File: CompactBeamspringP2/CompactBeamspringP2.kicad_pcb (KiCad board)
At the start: 2 copper layers, 163.6 x 33.2 mm, 68 parts, among them J1 BEAMSPRING CONNECTOR, J2 PadsToShort, J3 EXPANSION HEADER, U1 MCP4921-E, U2 LM339A, U3 74AHC595, U4 74AHC595, U5 ProMicro, U7 74AHC595

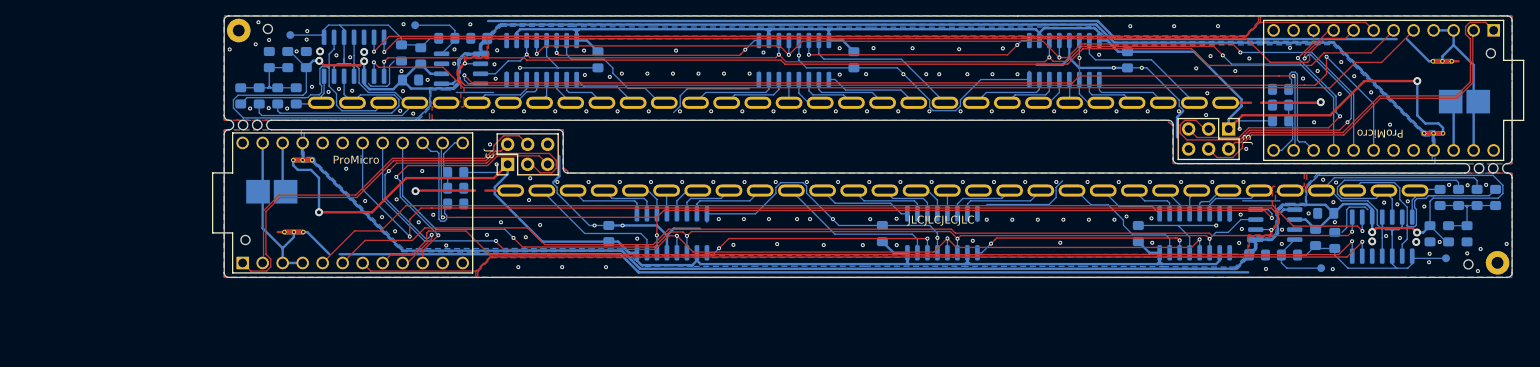
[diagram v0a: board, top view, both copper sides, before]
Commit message: Updated to rev. 1.4
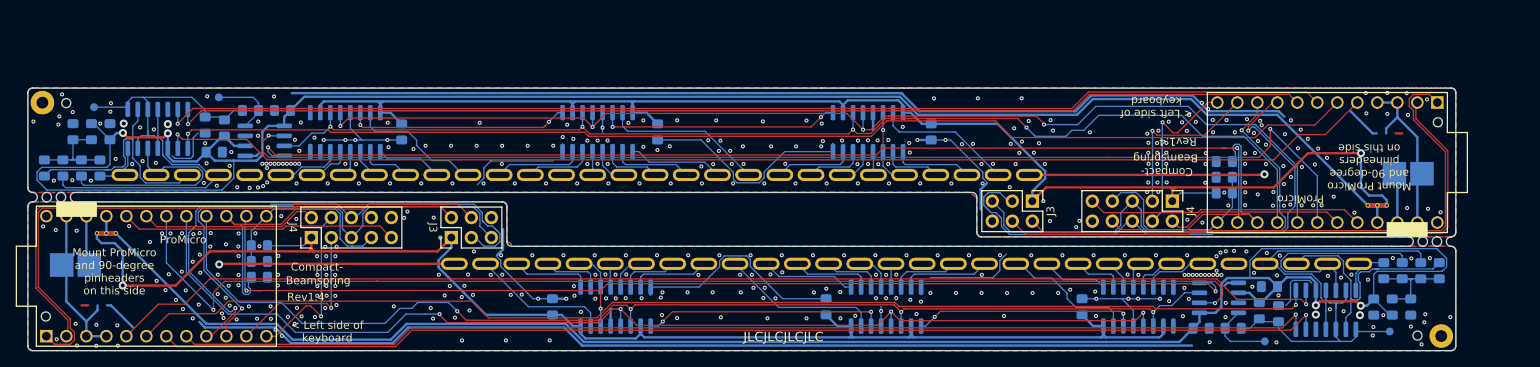
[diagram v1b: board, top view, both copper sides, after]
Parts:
- removed the C1 at (241.3, 128.8)
- removed the C1 at (142.4, 101.2)
- removed the C2 at (158.9, 126.0)
- removed the C2 at (224.8, 104.0)
- removed the C3 at (263.2, 126.1)
- removed the C3 at (120.5, 103.9)
- removed the C4 at (193.6, 126.0)
- removed the C4 at (190.0, 104.0)
- removed the C5 at (226.1, 126.0)
- removed the C5 at (157.5, 104.0)
- removed the C6 at (249.9, 123.5)
- removed the C6 at (133.7, 106.5)
- removed the H1 at (271.8, 129.8)
- removed the H1 at (111.9, 100.2)
- removed the J1 at (203.9, 120.6)
- removed the J1 at (179.8, 109.4)
- removed the J2 at (116.1, 117.8)
- removed the J2 at (267.6, 112.2)
- removed the J3 at (146.0, 117.2)
- removed the J3 at (237.6, 112.8)
- removed NT1 (x2): Net-Tie_3, NetTie:NetTie-3_THT_Pad0.3mm
- removed the NT2 at (118.8, 116.7)
- removed the NT2 at (264.8, 113.3)
- removed the R1 at (265.5, 126.1)
- removed the R1 at (118.1, 103.9)
- removed the R10 at (264.4, 121.5)
- removed the R10 at (119.2, 108.5)
- removed the R11 at (269.1, 121.5)
- removed the R11 at (114.5, 108.5)
- removed the R12 at (271.5, 121.5)
- removed the R12 at (112.2, 108.5)
- removed the R2 at (267.9, 126.1)
- removed the R2 at (115.8, 103.9)
- removed the R3 at (248.6, 126.5)
- removed the R3 at (135.0, 103.5)
- removed the R4 at (245.3, 128.8)
- removed the R4 at (138.3, 101.2)
- removed the R5 at (251.1, 126.9)
- removed the R5 at (132.6, 103.1)
- removed the R6 at (139.4, 118.3)
- removed the R6 at (244.2, 111.7)
- removed the R7 at (139.4, 120.3)
- removed the R7 at (244.2, 109.7)
- removed the R8 at (139.4, 122.3)
- removed the R8 at (244.2, 107.7)
- removed the R9 at (266.8, 121.5)
- removed the R9 at (116.8, 108.5)
- removed REF** (x4): tooling_hole, TH-XWhatsIt:tooling_hole
- removed the TP1 at (249.3, 130.4)
- removed the TP1 at (134.3, 99.6)
- removed the TP2 at (265.2, 129.2)
- removed the TP2 at (118.5, 100.8)
- removed the U1 at (243.5, 124.9)
- removed the U1 at (140.1, 105.1)
- removed the U2 at (257.1, 126.4)
- removed the U2 at (126.5, 103.6)
- removed the U3 at (166.9, 126.0)
- removed the U3 at (216.7, 104.0)
- removed the U4 at (201.3, 126.0)
- removed the U4 at (182.4, 104.0)
- removed the U5 at (126.4, 122.1)
- removed the U5 at (257.3, 107.9)
- removed the U7 at (233.3, 126.0)
- removed the U7 at (150.4, 104.0)
- added C1: 0U1, Capacitor_SMD:C_0805_2012Metric_Pad1.15x1.40mm_HandSolder, B.Cu at (234.1, 138.1)
- added C1: 0U1, Capacitor_SMD:C_0805_2012Metric_Pad1.15x1.40mm_HandSolder, B.Cu at (117.5, 110.4)
- added C2: 0U1, Capacitor_SMD:C_0805_2012Metric_Pad1.15x1.40mm_HandSolder, B.Cu at (151.7, 135.3)
- added C2: 0U1, Capacitor_SMD:C_0805_2012Metric_Pad1.15x1.40mm_HandSolder, B.Cu at (199.8, 113.1)
- added C3: 0U1, Capacitor_SMD:C_0805_2012Metric_Pad1.15x1.40mm_HandSolder, B.Cu at (256.0, 135.4)
- added C3: 0U1, Capacitor_SMD:C_0805_2012Metric_Pad1.15x1.40mm_HandSolder, B.Cu at (95.5, 113.1)
- added C4: 0U1, Capacitor_SMD:C_0805_2012Metric_Pad1.15x1.40mm_HandSolder, B.Cu at (186.5, 135.3)
- added C4: 0U1, Capacitor_SMD:C_0805_2012Metric_Pad1.15x1.40mm_HandSolder, B.Cu at (165.1, 113.1)
- added C5: 0U1, Capacitor_SMD:C_0805_2012Metric_Pad1.15x1.40mm_HandSolder, B.Cu at (219.0, 135.3)
- added C5: 0U1, Capacitor_SMD:C_0805_2012Metric_Pad1.15x1.40mm_HandSolder, B.Cu at (132.6, 113.1)
- added C6: 0U1, Capacitor_SMD:C_0805_2012Metric_Pad1.15x1.40mm_HandSolder, B.Cu at (242.8, 132.8)
- added C6: 0U1, Capacitor_SMD:C_0805_2012Metric_Pad1.15x1.40mm_HandSolder, B.Cu at (108.8, 115.7)
- added H1: MountingHole_Pad, TH-XWhatsIt:ChassisGnd, B.Cu at (264.6, 139.1)
- added H1: MountingHole_Pad, TH-XWhatsIt:ChassisGnd, B.Cu at (87.0, 109.4)
- added H2: ToolingHole, TH-XWhatsIt:tooling_hole, F.Cu at (87.4, 136.6)
- added H2: ToolingHole, TH-XWhatsIt:tooling_hole, F.Cu at (264.2, 111.9)
- added H3: ToolingHole, TH-XWhatsIt:tooling_hole, F.Cu at (261.6, 139.0)
- added H3: ToolingHole, TH-XWhatsIt:tooling_hole, F.Cu at (90.0, 109.5)
- added J1: BEAMSPRING CONNECTOR, TH-XWhatsIt:30-pin-universal-beamspring-connector_v2, F.Cu at (196.7, 129.9)
- added J1: BEAMSPRING CONNECTOR, TH-XWhatsIt:30-pin-universal-beamspring-connector_v2, F.Cu at (154.9, 118.6)
- added J2: PadsToShort, TH-XWhatsIt:PadsToShort, B.Cu at (91.2, 127.1)
- added J2: PadsToShort, TH-XWhatsIt:PadsToShort, B.Cu at (260.4, 121.3)
- added J3: EXPANSION HEADER, Connector_PinHeader_2.54mm:PinHeader_2x03_P2.54mm_Vertical, F.Cu at (138.9, 126.5)
- added J3: EXPANSION HEADER, Connector_PinHeader_2.54mm:PinHeader_2x03_P2.54mm_Vertical, F.Cu at (212.7, 121.9)
- added J4: Conn_02x05_Odd_Even, Connector_PinHeader_2.54mm:PinHeader_2x05_P2.54mm_Vertical, F.Cu at (121.1, 126.5)
- added J4: Conn_02x05_Odd_Even, Connector_PinHeader_2.54mm:PinHeader_2x05_P2.54mm_Vertical, F.Cu at (230.5, 121.9)
- added NT2: Net-Tie_3, NetTie:NetTie-3_THT_Pad0.3mm, B.Cu at (93.9, 126.0)
- added NT2: Net-Tie_3, NetTie:NetTie-3_THT_Pad0.3mm, B.Cu at (257.7, 122.5)
- added R1: 4K7, Resistor_SMD:R_0805_2012Metric_Pad1.15x1.40mm_HandSolder, B.Cu at (258.4, 135.4)
- added R1: 4K7, Resistor_SMD:R_0805_2012Metric_Pad1.15x1.40mm_HandSolder, B.Cu at (93.2, 113.1)
- added R10: 100k 1%, Resistor_SMD:R_0805_2012Metric_Pad1.15x1.40mm_HandSolder, B.Cu at (257.3, 130.8)
- added R10: 100k 1%, Resistor_SMD:R_0805_2012Metric_Pad1.15x1.40mm_HandSolder, B.Cu at (94.3, 117.7)
- added R11: 100k 1%, Resistor_SMD:R_0805_2012Metric_Pad1.15x1.40mm_HandSolder, B.Cu at (262.0, 130.8)
- added R11: 100k 1%, Resistor_SMD:R_0805_2012Metric_Pad1.15x1.40mm_HandSolder, B.Cu at (89.6, 117.7)
- added R12: 100k 1%, Resistor_SMD:R_0805_2012Metric_Pad1.15x1.40mm_HandSolder, B.Cu at (264.4, 130.8)
- added R12: 100k 1%, Resistor_SMD:R_0805_2012Metric_Pad1.15x1.40mm_HandSolder, B.Cu at (87.2, 117.7)
- added R2: 1K, Resistor_SMD:R_0805_2012Metric_Pad1.15x1.40mm_HandSolder, B.Cu at (260.7, 135.4)
- added R2: 1K, Resistor_SMD:R_0805_2012Metric_Pad1.15x1.40mm_HandSolder, B.Cu at (90.8, 113.1)
- added R3: 20K, Resistor_SMD:R_0805_2012Metric_Pad1.15x1.40mm_HandSolder, B.Cu at (241.5, 135.8)
- added R3: 20K, Resistor_SMD:R_0805_2012Metric_Pad1.15x1.40mm_HandSolder, B.Cu at (110.1, 112.6)
- added R4: 20K, Resistor_SMD:R_0805_2012Metric_Pad1.15x1.40mm_HandSolder, B.Cu at (238.2, 138.1)
- added R4: 20K, Resistor_SMD:R_0805_2012Metric_Pad1.15x1.40mm_HandSolder, B.Cu at (113.4, 110.4)
- added R5: 4K7, Resistor_SMD:R_0805_2012Metric_Pad1.15x1.40mm_HandSolder, B.Cu at (243.9, 136.2)
- added R5: 4K7, Resistor_SMD:R_0805_2012Metric_Pad1.15x1.40mm_HandSolder, B.Cu at (107.6, 112.3)
- added R6: Not Mounted, Resistor_SMD:R_0805_2012Metric_Pad1.15x1.40mm_HandSolder, B.Cu at (114.5, 127.6)
- added R6: Not Mounted, Resistor_SMD:R_0805_2012Metric_Pad1.15x1.40mm_HandSolder, B.Cu at (237.1, 120.9)
- added R7: Not Mounted, Resistor_SMD:R_0805_2012Metric_Pad1.15x1.40mm_HandSolder, B.Cu at (114.5, 129.6)
- added R7: Not Mounted, Resistor_SMD:R_0805_2012Metric_Pad1.15x1.40mm_HandSolder, B.Cu at (237.1, 118.9)
- added R8: Not Mounted, Resistor_SMD:R_0805_2012Metric_Pad1.15x1.40mm_HandSolder, B.Cu at (114.5, 131.6)
- added R8: Not Mounted, Resistor_SMD:R_0805_2012Metric_Pad1.15x1.40mm_HandSolder, B.Cu at (237.1, 116.9)
- added R9: 100k 1%, Resistor_SMD:R_0805_2012Metric_Pad1.15x1.40mm_HandSolder, B.Cu at (259.6, 130.8)
- added R9: 100k 1%, Resistor_SMD:R_0805_2012Metric_Pad1.15x1.40mm_HandSolder, B.Cu at (91.9, 117.7)
- added TP1: Dac Output, TestPoint:TestPoint_Pad_D1.0mm, B.Cu at (242.2, 139.7)
- added TP1: Dac Output, TestPoint:TestPoint_Pad_D1.0mm, B.Cu at (109.4, 108.7)
- added TP2: Threshold Voltage, TestPoint:TestPoint_Pad_D1.0mm, B.Cu at (258.1, 138.5)
- added TP2: Threshold Voltage, TestPoint:TestPoint_Pad_D1.0mm, B.Cu at (93.5, 110.0)
- added U1: MCP4921-E, Package_SO:SOIC-8_3.9x4.9mm_P1.27mm, B.Cu at (236.4, 134.2)
- added U1: MCP4921-E, Package_SO:SOIC-8_3.9x4.9mm_P1.27mm, B.Cu at (115.2, 114.3)
- added U2: LM339A, Package_SO:SOIC-14_3.9x8.7mm_P1.27mm, B.Cu at (250.0, 135.7)
- added U2: LM339A, Package_SO:SOIC-14_3.9x8.7mm_P1.27mm, B.Cu at (101.6, 112.7)
- added U3: 74AHC595, Package_SO:SOIC-16_3.9x9.9mm_P1.27mm, B.Cu at (159.8, 135.3)
- added U3: 74AHC595, Package_SO:SOIC-16_3.9x9.9mm_P1.27mm, B.Cu at (191.8, 113.2)
- added U4: 74AHC595, Package_SO:SOIC-16_3.9x9.9mm_P1.27mm, B.Cu at (194.1, 135.3)
- added U4: 74AHC595, Package_SO:SOIC-16_3.9x9.9mm_P1.27mm, B.Cu at (157.5, 113.2)
- added U5: ProMicro, promicro:ProMicro, F.Cu at (101.4, 131.4)
- added U5: ProMicro, promicro:ProMicro, F.Cu at (250.1, 117.0)
- added U7: 74AHC595, Package_SO:SOIC-16_3.9x9.9mm_P1.27mm, B.Cu at (226.1, 135.3)
- added U7: 74AHC595, Package_SO:SOIC-16_3.9x9.9mm_P1.27mm, B.Cu at (125.4, 113.2)
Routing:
- net GND: track 44.3 -> 546.5 mm, vias 0 -> 482
- net GNDA: track 262.6 -> 0.00 mm, vias 60 -> 0
- net GNDD: track 221.8 -> 0.00 mm, vias 146 -> 0
- net HEADER1_LED5: track 0.00 -> 140.0 mm, vias 0 -> 2
- net HEADER2_LED4: track 0.00 -> 128.7 mm, vias 0 -> 2
- net HEADER1: track 90.4 -> 0.00 mm, vias 4 -> 0
- net BUTTON2: track 0.00 -> 70.4 mm
- net BUTTON3: track 0.00 -> 70.2 mm
- net HEADER2: track 69.5 -> 0.00 mm, vias 4 -> 0
- net HEADER3: track 92.5 -> 152.5 mm
- net HEADER4: track 89.8 -> 148.0 mm
- net BUTTON1: track 0.00 -> 50.3 mm
- net LED1: track 0.00 -> 45.2 mm
- net LED3: track 0.00 -> 44.4 mm, vias 0 -> 2
- net LED2: track 0.00 -> 43.3 mm, vias 0 -> 2
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- added copper zone on B.Cu, net GND
- added copper zone on F.Cu, net GND
- removed copper zone on B.Cu, net GNDA
- removed copper zone on F.Cu, net GNDA
- removed copper zone on B.Cu, net GNDD
- removed copper zone on F.Cu, net GNDD
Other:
- board size 163.6 x 33.2 mm -> 181.3 x 33.3 mm
- board text added: "+5V"
- board text added: "< Left side of keyboard"
- board text added: "BTNs"
- board text added: "Beamspring"
- board text added: "Compact-"
- board text added: "Compact-Beamspring Rev1.4"
- board text added: "EN"
- board text added: "Expansion Header e.g. Solenoid Drv."
- board text added: "LEDs no res"
- board text added: "Left side of > keyboard"
- board text added: "More Expansion e.g. 3278 extra leds+buttons"
- board text added: "Mount ProMicro and 90-degree pinheaders on this side"
- board text added: "Rev1.4"
- board text added: "TRIG"
- board text removed: "Compact-Beamspring Rev1.3"
